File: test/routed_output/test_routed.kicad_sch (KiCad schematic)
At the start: 6 parts, among them U1 R_0805_2012Metric_Pad1.20x1.4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, U2 SOT-23, U3 TO-220-3_Horizontal_TabDown, U4 TO-92_Wide, U5 R_Axial_DIN0207_L6.3mm_D2.5mm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, U6 R_Axial_DIN0207_L6.3mm_D2.5mm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

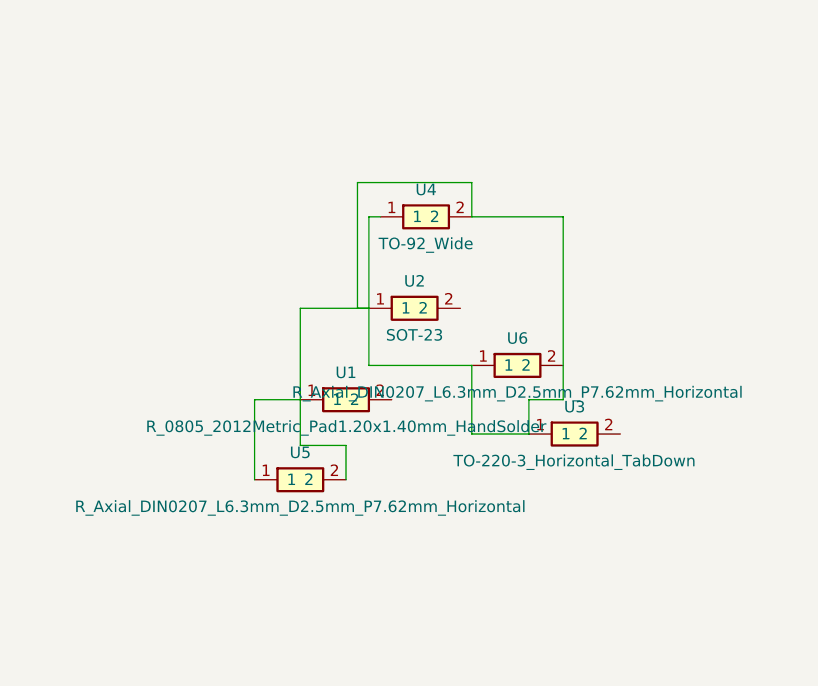
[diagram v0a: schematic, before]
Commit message: backup
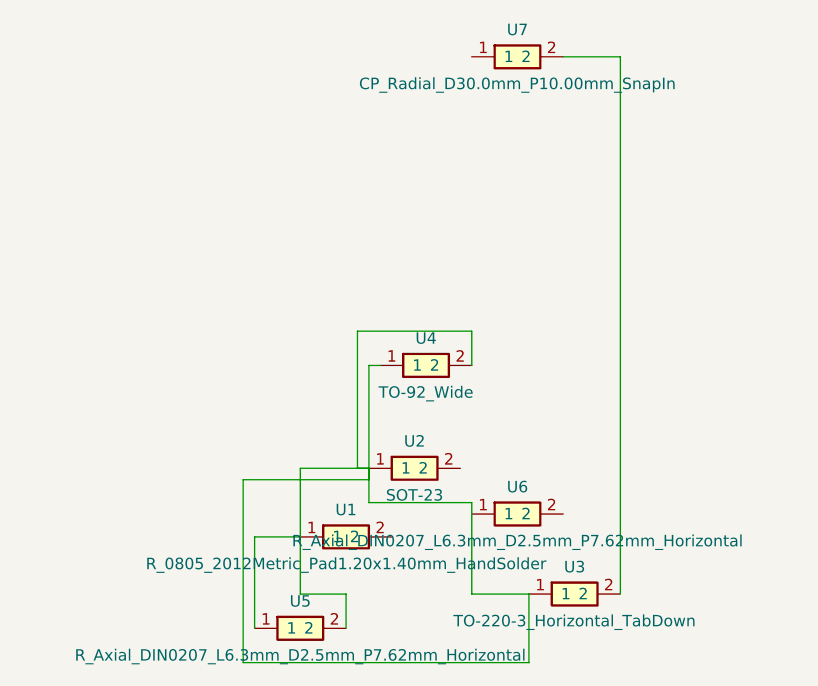
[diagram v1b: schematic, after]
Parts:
- added U7: CP_Radial_D30.0mm_P10.00mm_SnapIn, RE_passive_tht:CP_Radial_D30.0mm_P10.00mm_SnapIn, symbol RE_passive:C_Polarized
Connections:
- net at U1.1, U2.1, U3.1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: no longer U6.1
- net at U3.2: now also U7.2
